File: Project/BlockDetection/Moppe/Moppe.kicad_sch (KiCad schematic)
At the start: 12 parts, among them J1 Conn_01x03_Pin, J2 Conn_01x02_Pin, J3 Conn_01x02_Pin, Q1 BC856 or BC557, U1 PC817

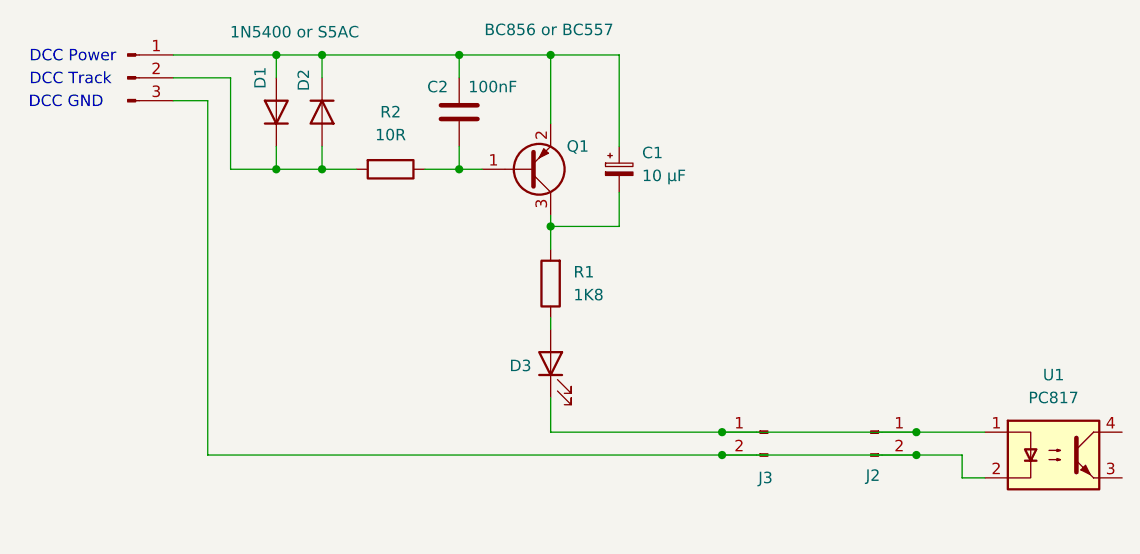
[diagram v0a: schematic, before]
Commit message: SporBesat a la´ Moppe
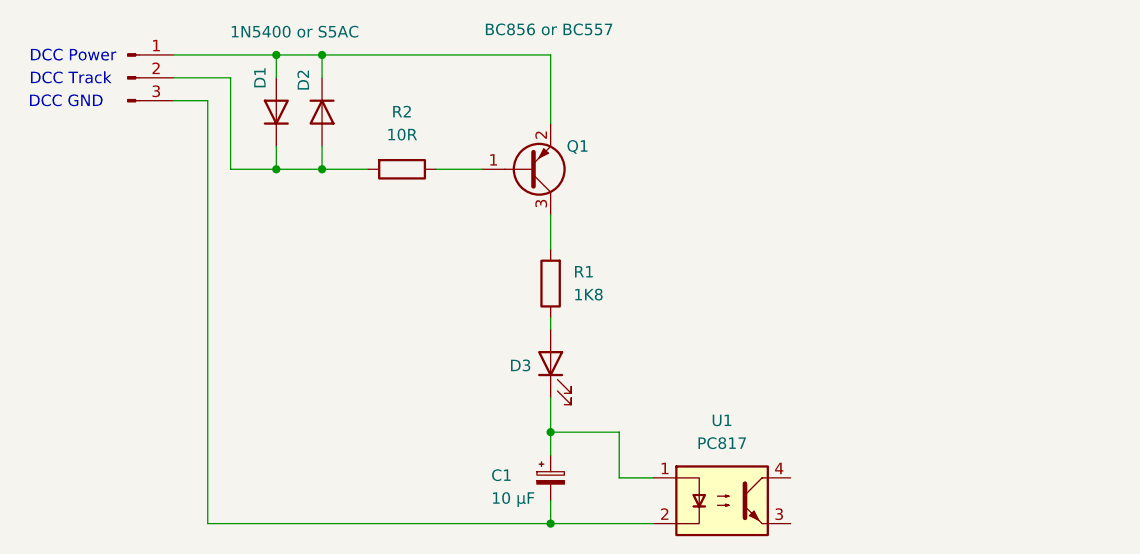
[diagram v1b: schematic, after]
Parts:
- removed C2: 100nF, symbol Device:C
- removed J2, J3: Conn_01x02_Pin, symbol Connector:Conn_01x02_Pin
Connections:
- net at Q1.3 (C), R1.2: no longer C1.2
- net at D3.1 (K), U1.1: now also C1.1
- net at J1.3 (Pin_3), U1.2: now also C1.2
- net at D1.2 (A), D2.1 (K), J1.1 (Pin_1)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: no longer C1.1
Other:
- moved on the sheet: C1, R2, U1
